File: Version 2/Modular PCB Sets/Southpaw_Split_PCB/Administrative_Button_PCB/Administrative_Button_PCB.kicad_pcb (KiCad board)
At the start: 2 copper layers, 163 x 27 mm, 17 parts, among them J1 Conn_01x07_Socket

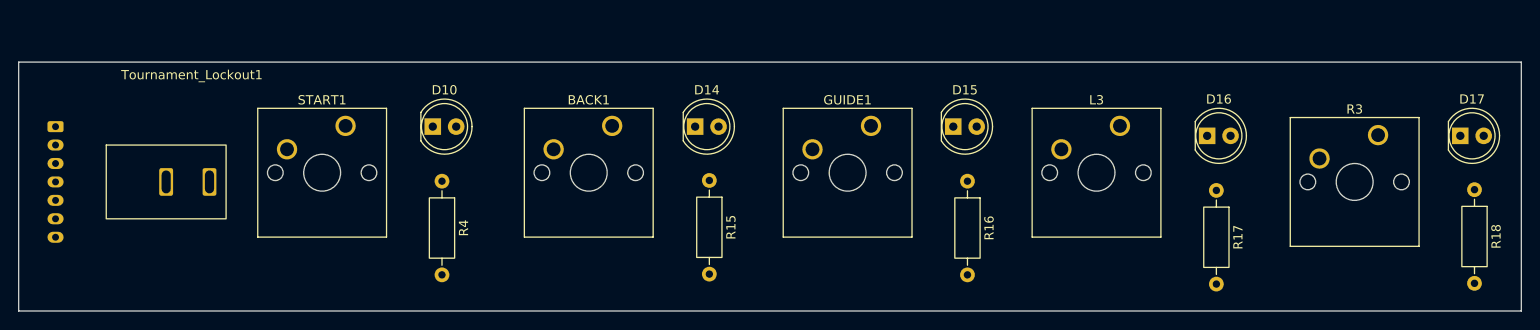
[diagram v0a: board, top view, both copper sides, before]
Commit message: general part layout
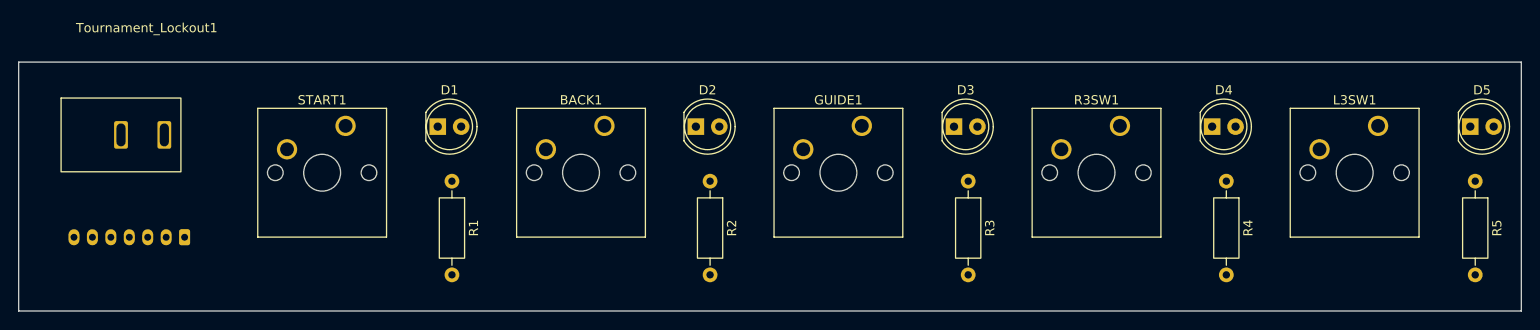
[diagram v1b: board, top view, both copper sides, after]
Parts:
- removed D10, D14, D15, D16, D17: LED, LED_THT:LED_D5.0mm
- removed L3: SW_SPST, Button_Switch_Keyboard:SW_Cherry_MX_1.00u_PCB
- removed R15, R16, R17, R18: R, Resistor_THT:R_Axial_DIN0207_L6.3mm_D2.5mm_P10.16mm_Horizontal
- added D1: LED, LED_THT:LED_D5.0mm, F.Cu at (63.5, 126.0)
- added D2: LED, LED_THT:LED_D5.0mm, F.Cu at (91.5, 126.0)
- added D3: LED, LED_THT:LED_D5.0mm, F.Cu at (119.5, 126.0)
- added D4: LED, LED_THT:LED_D5.0mm, F.Cu at (147.5, 126.0)
- added D5: LED, LED_THT:LED_D5.0mm, F.Cu at (175.5, 126.0)
- added L3SW1: SW_SPST, Button_Switch_Keyboard:SW_Cherry_MX_1.00u_PCB, F.Cu at (165.5, 125.9)
- added R1: R, Resistor_THT:R_Axial_DIN0207_L6.3mm_D2.5mm_P10.16mm_Horizontal, F.Cu at (65.0, 131.9)
- added R2: R, Resistor_THT:R_Axial_DIN0207_L6.3mm_D2.5mm_P10.16mm_Horizontal, F.Cu at (93.0, 131.9)
- added R3SW1: SW_SPST, Button_Switch_Keyboard:SW_Cherry_MX_1.00u_PCB, F.Cu at (137.5, 125.9)
- added R5: R, Resistor_THT:R_Axial_DIN0207_L6.3mm_D2.5mm_P10.16mm_Horizontal, F.Cu at (176.0, 131.9)
- R3: value SW_SPST -> R; footprint Button_Switch_Keyboard:SW_Cherry_MX_1.00u_PCB -> Resistor_THT:R_Axial_DIN0207_L6.3mm_D2.5mm_P10.16mm_Horizontal
- moved R4 85.1 mm to (149.0, 131.9)
- moved R3 44.7 mm to (121.0, 131.9), turned to -90 degrees
- moved J1 18.4 mm to (36.0, 138.0), turned to 180 degrees
- moved Tournament_Lockout1 7.07 mm to (22.6, 130.9)
- moved GUIDE1 1.00 mm to (109.5, 125.9)
- moved BACK1 0.84 mm to (81.5, 125.9)
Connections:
- R3 pad 1: /R3 -> Net-(D3-A)
- R3 pad 2: Net-(BACK1-B) -> /3V3

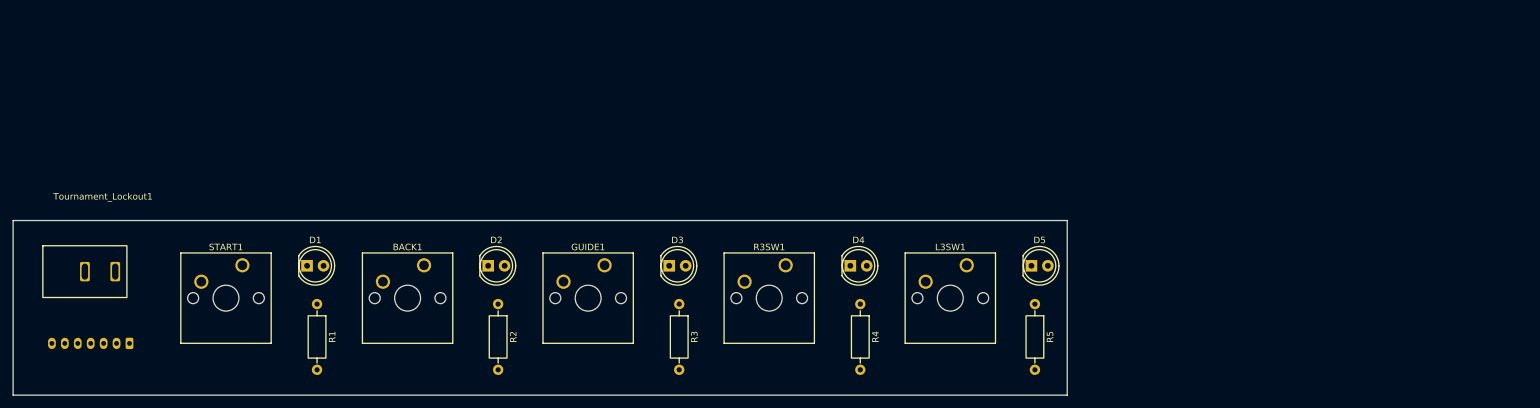
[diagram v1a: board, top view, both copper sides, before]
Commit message: Finalized design and uploaded gerbers to JLCpcb, waiting for boards to come in
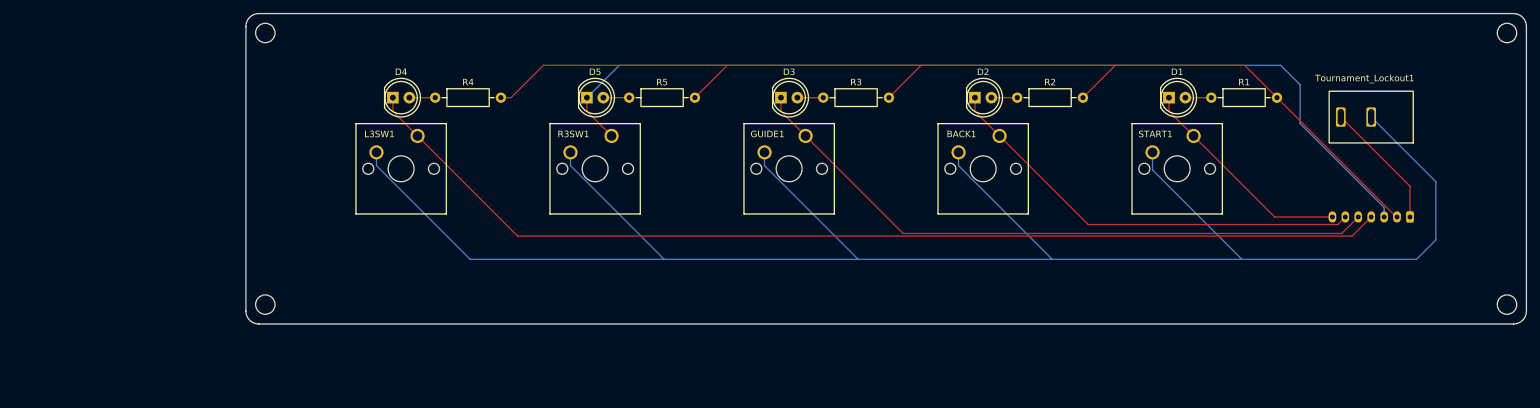
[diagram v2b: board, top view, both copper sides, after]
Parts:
- moved Tournament_Lockout1 214.3 mm to (234.5, 99.0), turned to 180 degrees
- moved J1 199.0 mm to (234.0, 118.5)
- moved START1 148.4 mm to (200.5, 105.9)
- moved R1 141.9 mm to (203.3, 100.0), turned to 0 degrees
- moved D1 135.8 mm to (196.7, 100.0)
- moved BACK1 91.2 mm to (170.5, 105.9)
- moved L3SW1 87.2 mm to (80.5, 105.9)
- moved R2 86.4 mm to (173.3, 100.0), turned to 0 degrees
- moved D2 79.6 mm to (166.7, 100.0)
- moved D4 75.4 mm to (76.7, 100.0)
- moved D5 73.5 mm to (106.7, 100.0)
- moved R4 73.1 mm to (83.3, 100.0), turned to 0 degrees
- moved R5 70.4 mm to (113.3, 100.0), turned to 0 degrees
- moved R3 38.9 mm to (143.3, 100.0), turned to 0 degrees
- moved GUIDE1 37.0 mm to (140.5, 105.9)
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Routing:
- net Net-(BACK1-B): track 0.00 -> 286.1 mm
- net /3V3: track 0.00 -> 172.1 mm
- net /L3: track 0.00 -> 162.6 mm
- net /R3: track 0.00 -> 146.9 mm
- net /Guide: track 0.00 -> 100.3 mm
- net /Options: track 0.00 -> 67.1 mm
- net /Start: track 0.00 -> 34.1 mm
- net /Gnd: track 0.00 -> 19.9 mm
- net Net-(D5-A): track 0.00 -> 4.00 mm
- net Net-(D4-A): track 0.00 -> 4.00 mm
- net Net-(D3-A): track 0.00 -> 4.00 mm
- net Net-(D2-A): track 0.00 -> 4.00 mm
- net Net-(D1-A): track 0.00 -> 4.00 mm
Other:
- board size 163 x 27 mm -> 198 x 48 mm
